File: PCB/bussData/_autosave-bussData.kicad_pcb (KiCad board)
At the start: 2 copper layers, 7 parts

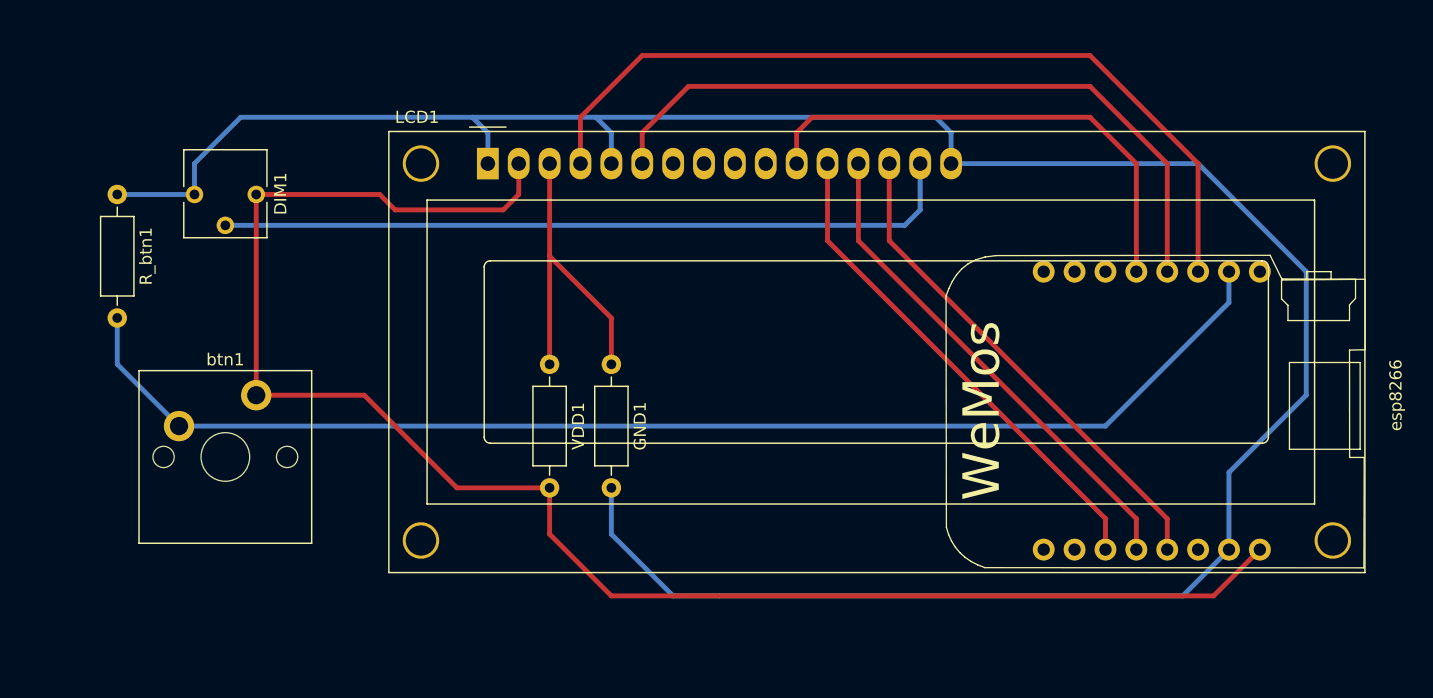
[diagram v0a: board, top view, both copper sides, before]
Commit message: updated pcb
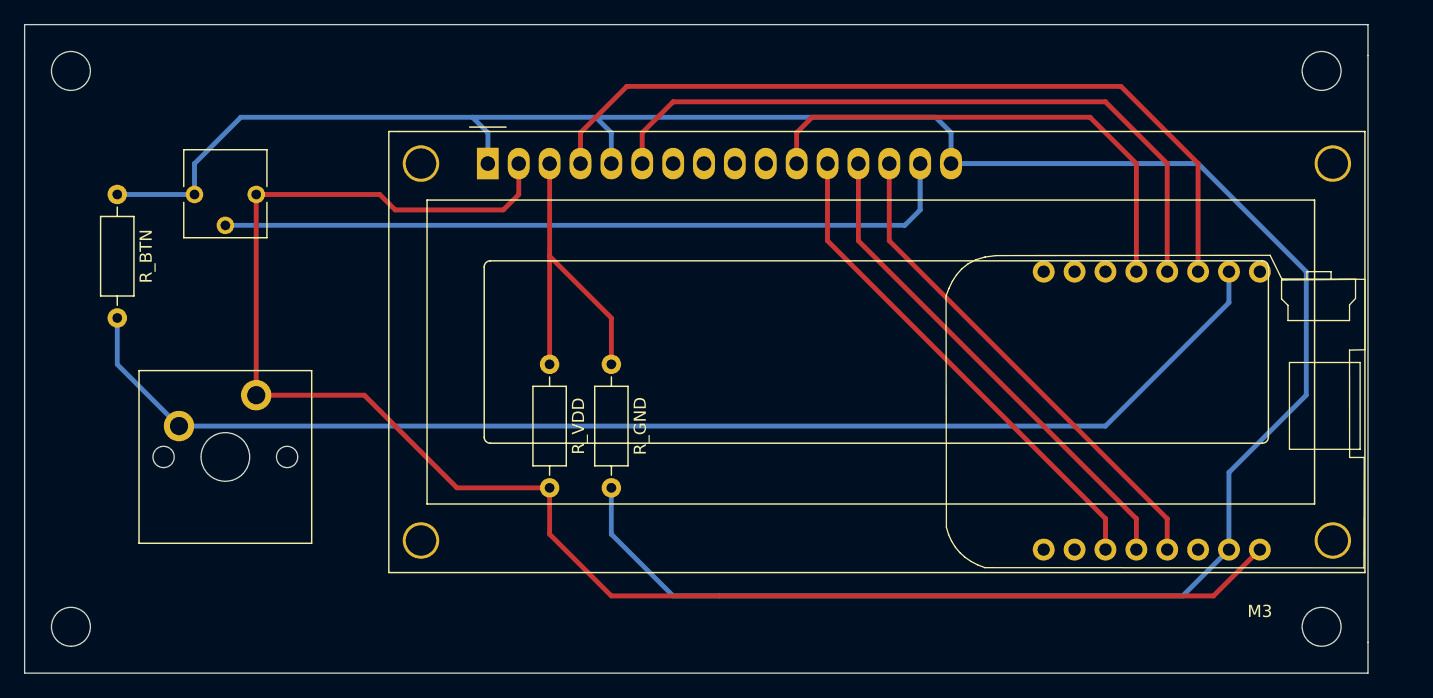
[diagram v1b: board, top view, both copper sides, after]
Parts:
- added M3: MountingHole_3.2mm_M3, MountingHole:MountingHole_3.2mm_M3, F.Cu at (184.2, 104.1)
- added REF**: MountingHole_3.2mm_M3, MountingHole:MountingHole_3.2mm_M3, F.Cu at (81.3, 104.1)
- added REF**: MountingHole_3.2mm_M3, MountingHole:MountingHole_3.2mm_M3, F.Cu at (81.3, 58.4)
- added REF**: MountingHole_3.2mm_M3, MountingHole:MountingHole_3.2mm_M3, F.Cu at (184.2, 58.4)
- esp8266 D1 Wemos mini: renamed from esp8266
- renumbered R_btn1 to R_BTN, GND1 to R_GND, VDD1 to R_VDD
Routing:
- net Net-(LCD1-Pad4): track 69.3 -> 66.4 mm
- net Net-(LCD1-Pad6): track 58.8 -> 57.8 mm
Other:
- board outline added: 110.5 x 53.3 mm
- board text added: "By Anders Mørk"
